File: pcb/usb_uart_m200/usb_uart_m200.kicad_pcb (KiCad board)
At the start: 2 copper layers, 25.2 x 25.2 mm, 17 parts, among them J1 Conn_01x02_Socket, P1 USB_C_Plug_USB2.0, U1 CY7C65213-28PVXI, U2 MIC5317-3.3xM5, U4 USBLC6-2SC6, X1 2059-301_998-403

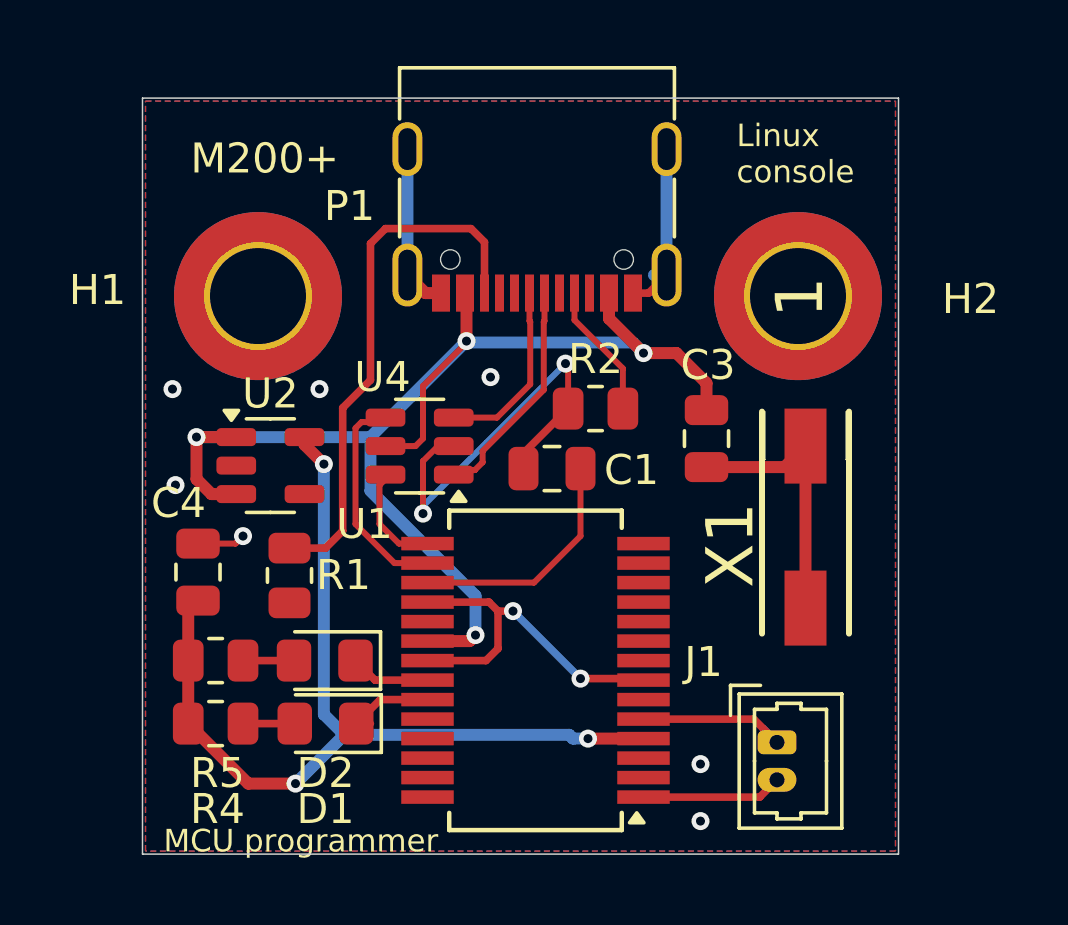
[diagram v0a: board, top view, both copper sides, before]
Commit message: PCB sources after production
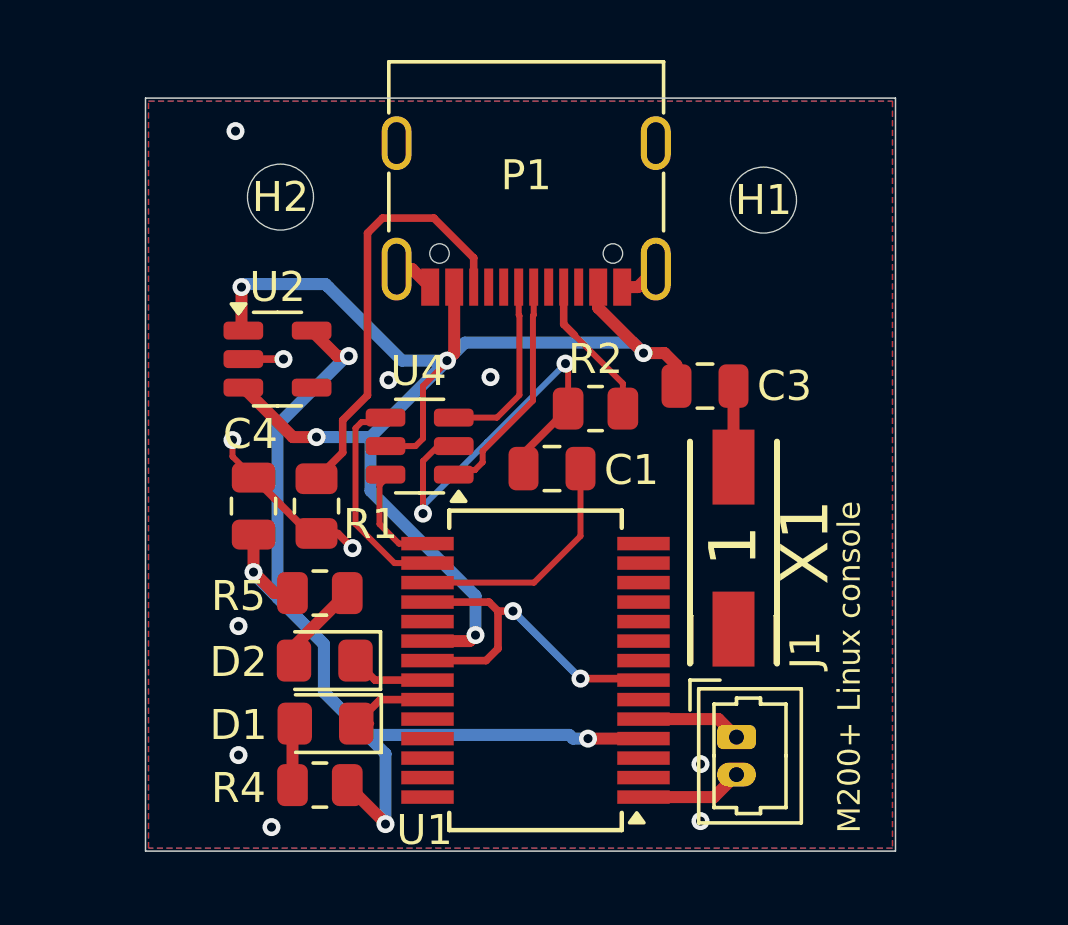
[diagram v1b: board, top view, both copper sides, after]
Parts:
- H1, H2: footprint MountingHole:MountingHole_3.2mm_M3_DIN965_Pad_TopBottom -> MountingHole:MountingHole_2.2mm_M2_ISO7380
- moved H2 17.6 mm to (151.5, 57.2)
- moved H1 17.2 mm to (167.6, 57.3)
- moved R5 4.14 mm to (152.8, 70.4)
- moved R4 4.03 mm to (152.8, 76.8), turned to 180 degrees
- moved U2 3.56 mm to (151.4, 62.6)
- moved C4 2.87 mm to (150.6, 67.5)
- moved R1 2.48 mm to (152.7, 67.5)
- moved X1 2.46 mm to (166.6, 68.8), turned to -90 degrees
- moved C3 1.75 mm to (165.7, 63.5), turned to 0 degrees
- moved J1 1.36 mm to (166.7, 75.2)
- moved P1 0.41 mm to (159.7, 56.5)
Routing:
- net GND: track 49.0 -> 38.7 mm, vias 11 -> 15
- net /3v3: track 31.6 -> 39.2 mm, vias 3 -> 4
- net Net-(P1-VCONN): track 17.9 -> 14.2 mm
- net /VBUS: track 43.2 -> 46.3 mm, vias 4 -> 5
- net /MCU/CON_TX_PC_RX: track 5.44 -> 3.35 mm
- net Net-(D2-A): track 1.70 -> 2.99 mm
- net /MCU/CON_RX_PC_TX: track 4.69 -> 3.41 mm
- net Net-(D1-A): track 1.72 -> 2.35 mm
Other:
- board size 25.2 x 25.2 mm -> 25 x 25.1 mm
- board text added: "M200+ Linux console"
- board text removed: "Linux console"
- board text removed: "M200+"
- board text removed: "MCU programmer"
